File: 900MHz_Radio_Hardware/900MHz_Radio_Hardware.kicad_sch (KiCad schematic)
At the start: 18 parts, among them SW1 SW_SPDT, U1 TSR_1-2450

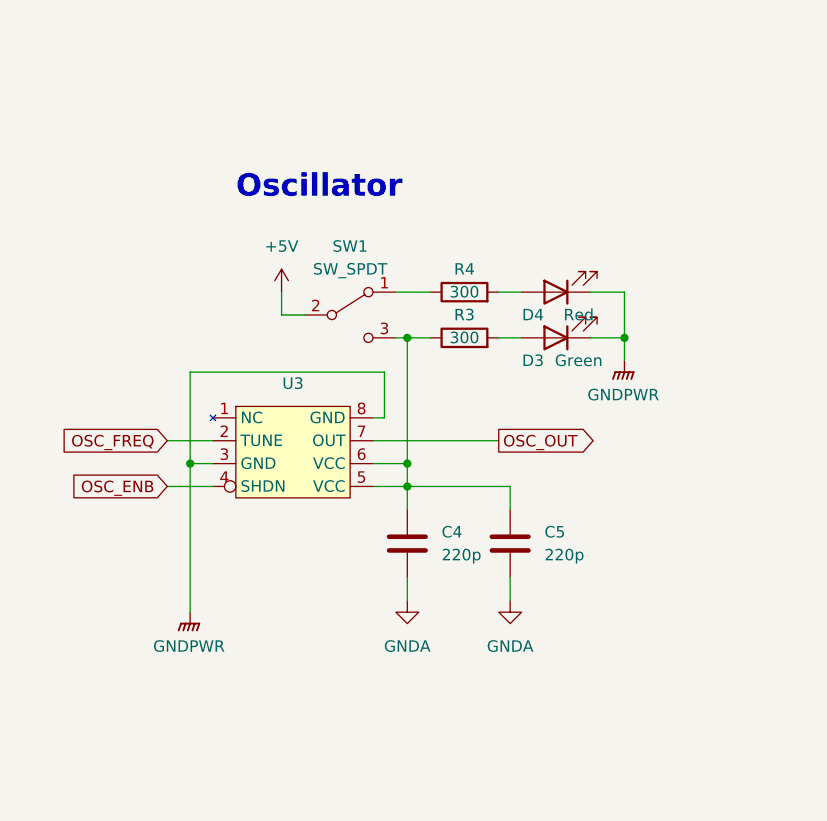
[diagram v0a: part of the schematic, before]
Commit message: Updated filter
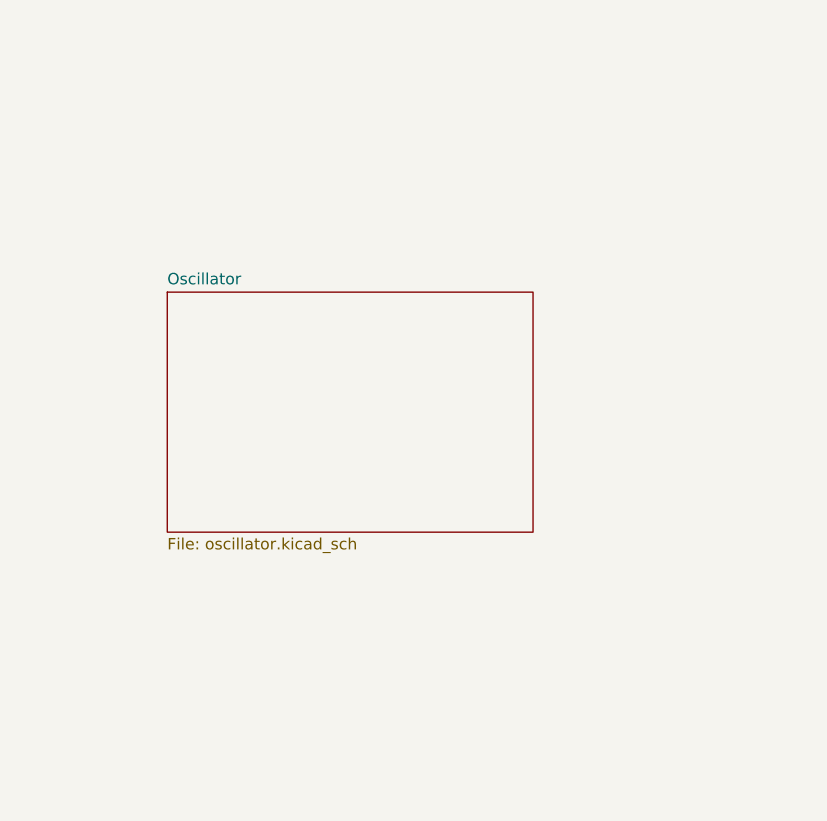
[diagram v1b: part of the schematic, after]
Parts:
- removed C4, C5: 220p, symbol Device:C
- removed D3: Green, symbol Device:LED
- removed D4: Red, symbol Device:LED
- removed R3, R4: 300, symbol Device:R
- removed SW1: SW_SPDT, symbol Switch:SW_SPDT
- removed U3: ~, Package_SO:MSOP-8_3x3mm_P0.65mm, symbol MRDT_ICs:MAX2623EUA+T
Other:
- added sheet Oscillator (oscillator.kicad_sch)
- note removed: "Oscillator"
